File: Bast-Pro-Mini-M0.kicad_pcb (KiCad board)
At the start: 2 copper layers, 17.8 x 33 mm, 24 parts, among them J1 USB_B_Micro, J2 Conn_02x02_Odd_Even, P1 Digital, P2 ADC, P3 Analog, U1 AP2112K-3.3TRG1, U2 ATSAMD21E18A-AF

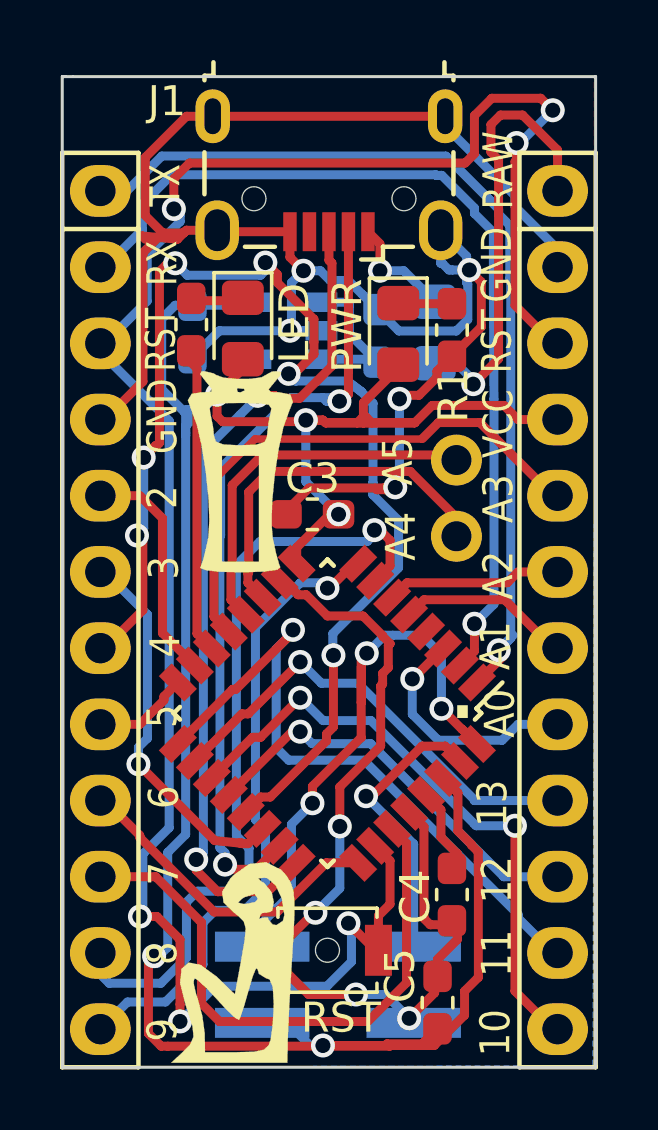
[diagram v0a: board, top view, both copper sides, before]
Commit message: Update tracks
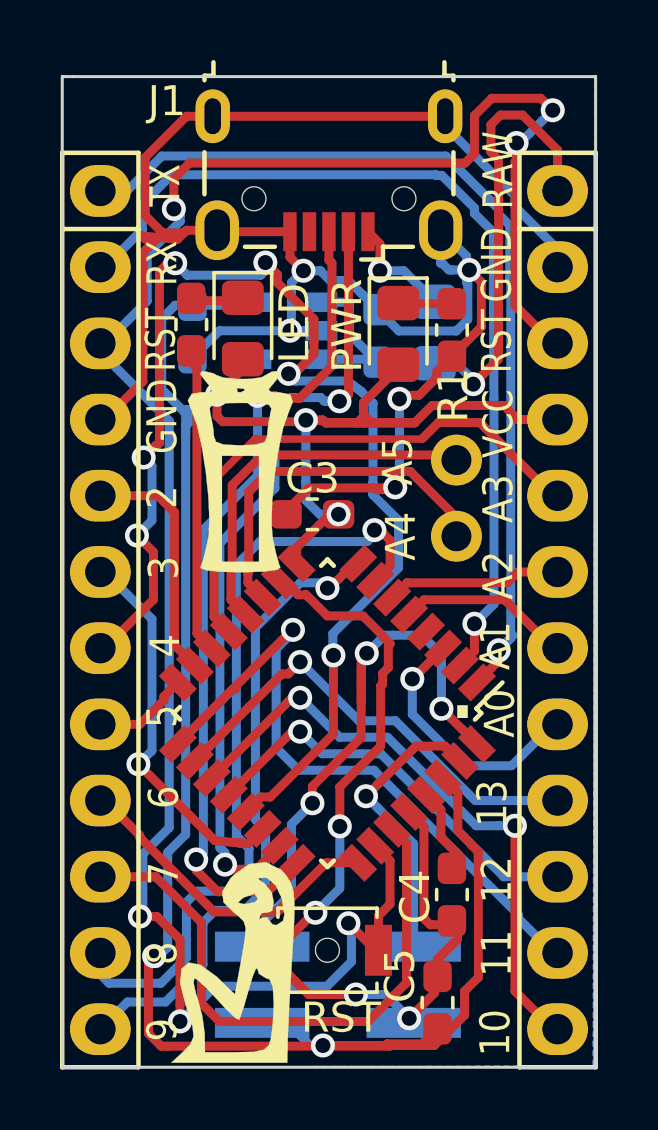
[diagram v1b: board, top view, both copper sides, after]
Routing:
- net /11(**/MOSI): track 22.2 -> 24.7 mm
- net /A0: track 8.04 -> 8.75 mm
- net /D+: track 28.5 -> 29.2 mm
- net /4: track 42.9 -> 43.4 mm
